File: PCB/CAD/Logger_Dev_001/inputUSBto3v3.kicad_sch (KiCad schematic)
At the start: 22 parts, among them J4 Connector, USB-TYPE-C-16P, U4 MCP2221AxSL, U6 XC6206P332MR

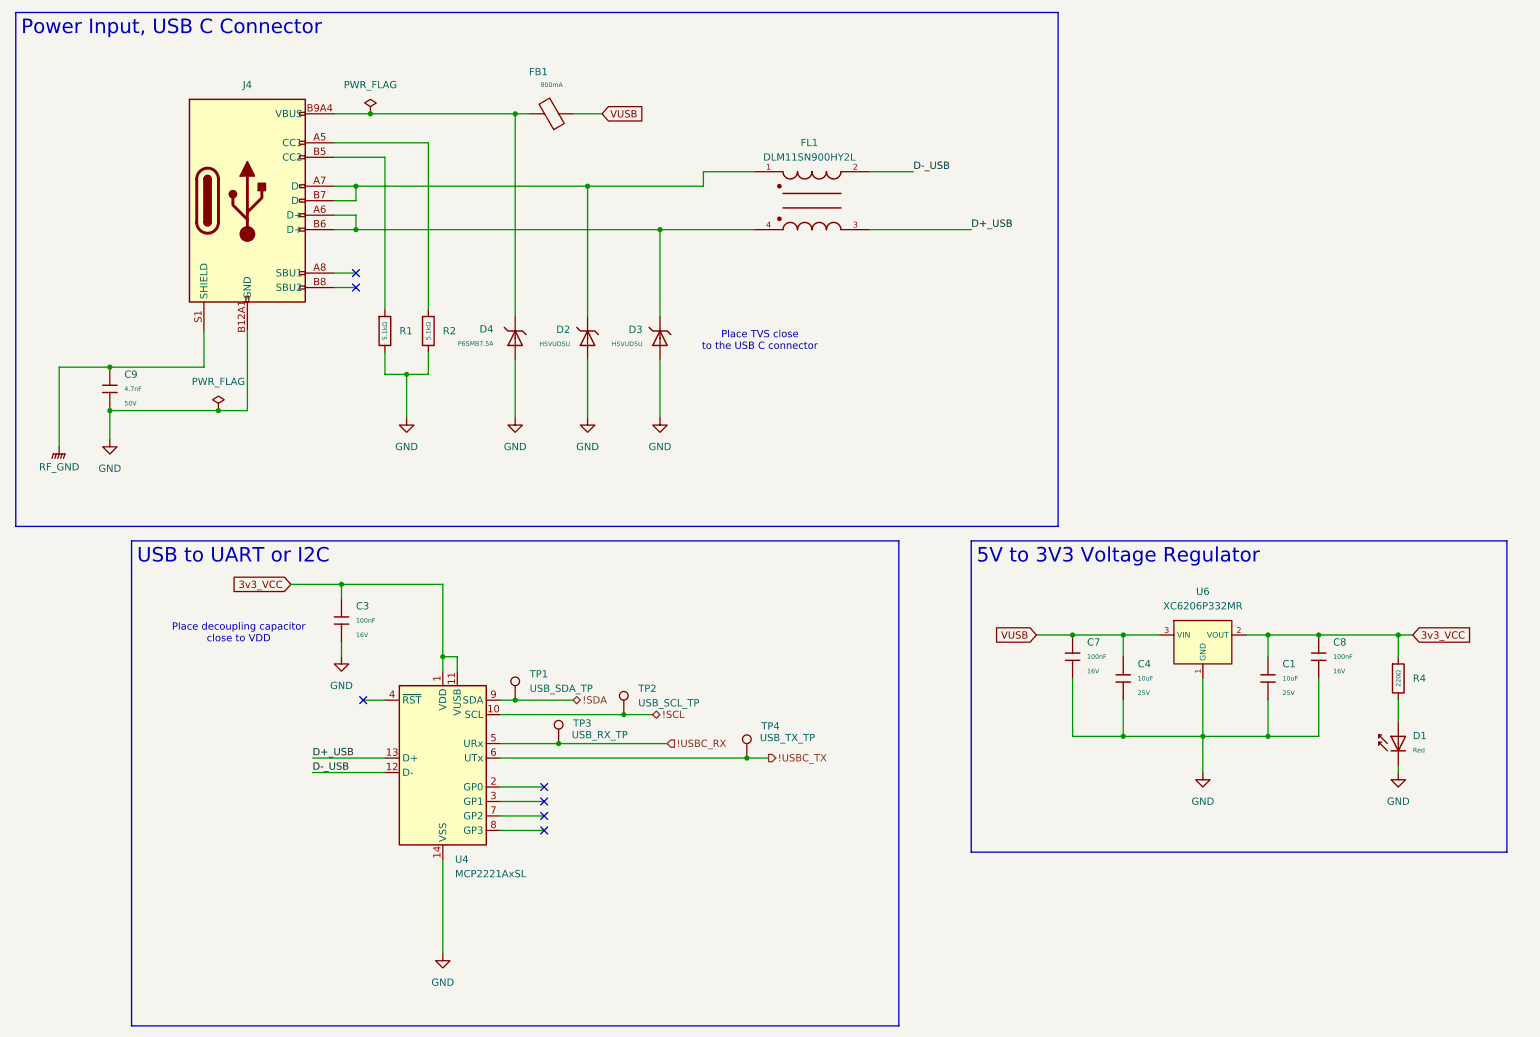
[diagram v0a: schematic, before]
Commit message: Updated Schematic
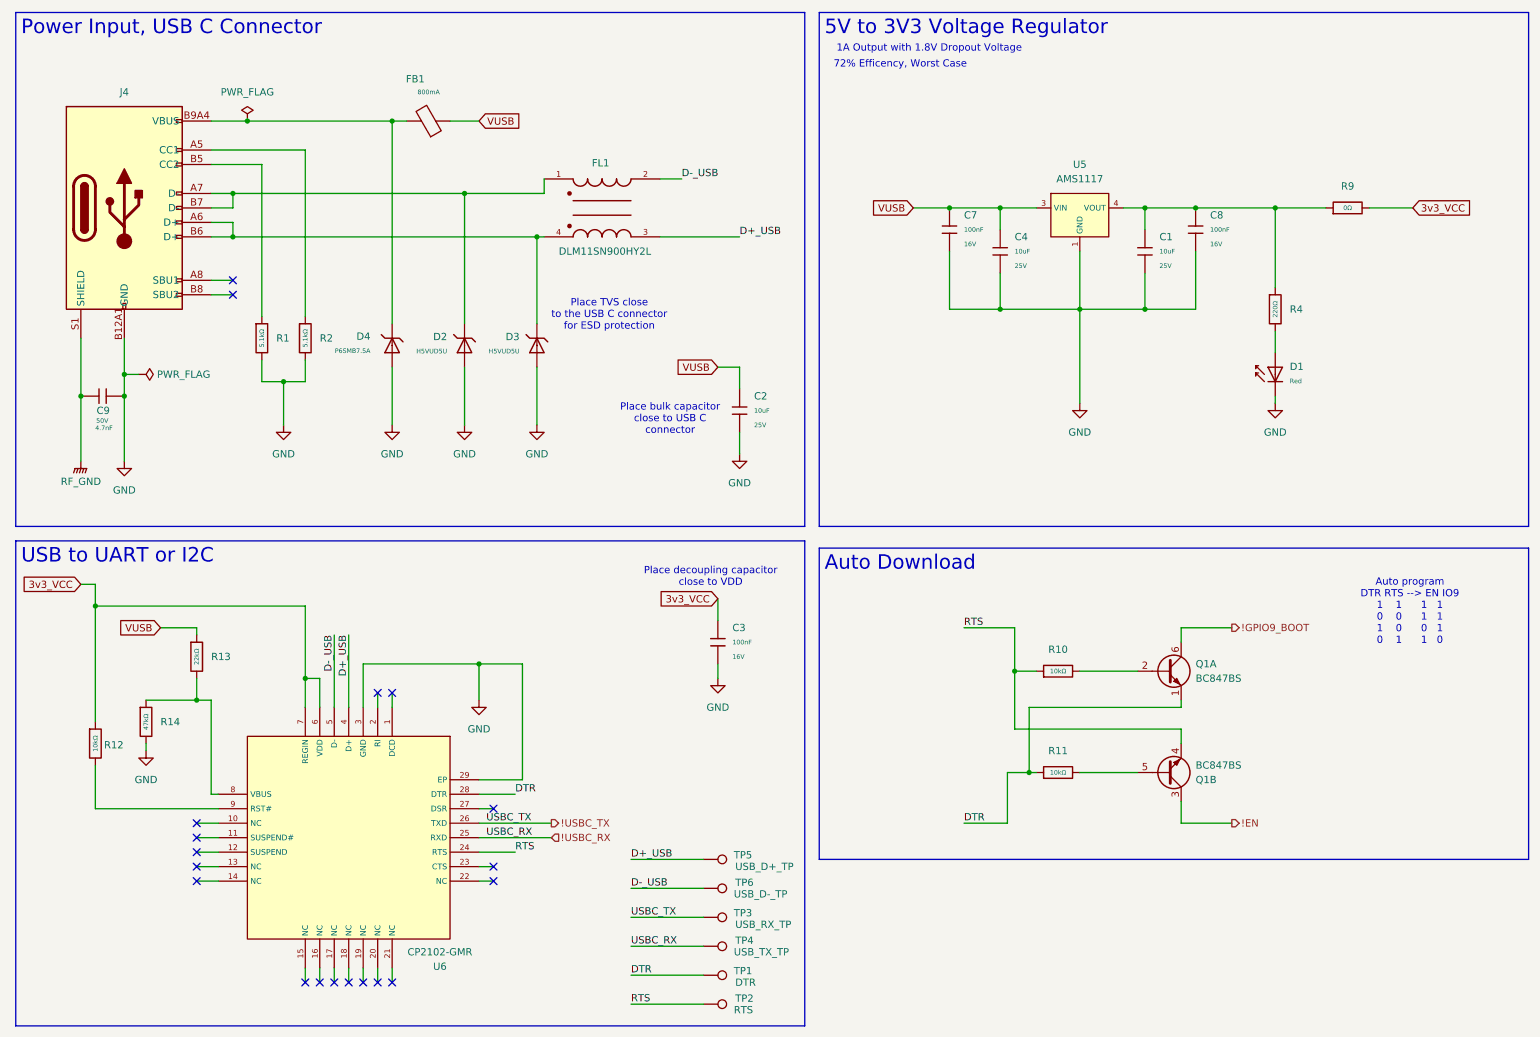
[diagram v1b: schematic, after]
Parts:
- removed U4: MCP2221AxSL, Package_SO:SOIC-14_3.9x8.7mm_P1.27mm, symbol Interface_USB:MCP2221AxSL
- removed U6: XC6206P332MR, PCM_JLCPCB:SOT-23-3_L2.9-W1.6-P1.90-LS2.8-BR, symbol PCM_JLCPCB-Power:LDO, 3.3V, 0.2A
- added C2: 10uF, PCM_JLCPCB:C_0603, symbol PCM_JLCPCB-Capacitors:0603,10uF,(2)
- added Q1: BC847BS, PCM_JLCPCB:SOT-363_SC-70-6, symbol PCM_JLCPCB-Transistor-Packages:NPN, 2 Channel, BC847BS
- added R10, R11, R12: 10kΩ, PCM_JLCPCB:R_0402, symbol PCM_JLCPCB-Resistors:0402,10kΩ
- added R13: 22kΩ, PCM_JLCPCB:R_0402, symbol PCM_JLCPCB-Resistors:0402,22kΩ
- added R14: 47kΩ, PCM_JLCPCB:R_0402, symbol PCM_JLCPCB-Resistors:0402,47kΩ
- added R9: 0Ω, PCM_JLCPCB:R_1206, symbol PCM_JLCPCB-Resistors:1206,0Ω
- added TP5: USB_D+_TP, symbol Connector:TestPoint
- added TP6: USB_D-_TP, symbol Connector:TestPoint
- added U5: AMS1117, PCM_JLCPCB:SOT-223-3_L6.5-W3.4-P2.30-LS7.0-BR, symbol PCM_JLCPCB-Power:LDO, 3.3V, 1A
- added U6: CP2102-GMR, PCM_JLCPCB:WQFN-28_L5.0-W5.0-P0.50-BL-EP3.2, symbol PCM_JLCPCB-Interface:Transceiver, USB
- TP1: value USB_SDA_TP -> DTR
- TP2: value USB_SCL_TP -> RTS
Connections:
- net !USBC_RX: now also TP4.1, U6.25 (RXD); no longer TP3.1
- net !USBC_TX: now also TP3.1, U6.26 (TXD); no longer TP4.1
- net 3v3_VCC: now also R12.1, R9.2, U6.6 (VDD), U6.7 (REGIN); no longer C1.1, C8.1, R4.1
- net D+_USB: now also TP5.1, U6.4 (D+)
- net D-_USB: now also TP6.1, U6.5 (D-)
- net GND: now also C2.2, R14.2, U5.1 (GND), U6.29 (EP), U6.3 (GND)
- net VUSB: now also C2.1, R13.1, U5.3 (VIN)
- net !SCL renamed RTS
- net RTS: now also Q1.4 (E2), R10.1, U6.24 (RTS)
- net !SDA renamed DTR
- net DTR: now also Q1.1 (E1), R11.1, U6.28 (DTR)
- new net: C1.1, C8.1, R4.1, R9.1, U5.2 (VOUT), U5.4 (VOUT)
- new net: Q1.2 (B1), R10.2
- new net: R12.2, U6.9 (RST#)
- new net: R13.2, R14.1, U6.8 (VBUS)
- new net: Q1.5 (B2), R11.2
- new net !EN: Q1.3 (C2)
- new net !GPIO9_BOOT: Q1.6 (C1)
- no-connect marks 7 -> 19
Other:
- note added: "1A Output with 1.8V Dropout Voltage"
- note added: "72% Efficency, Worst Case"
- note added: "Auto program DTR RTS --> EN IO9 1 1 1 1 0 0 1 1 1 0 0 1 0 1 1 0"
- note added: "Place TVS close to the USB C connector for ESD protection"
- note added: "Place bulk capacitor close to USB C connector"
- note removed: "Place TVS close to the USB C connector"
- company: (none) -> Jake Odgers
- title: (none) -> Mileage Logger
- moved on the sheet: C1, C3, C4, C7, C8, C9, D1, D2, D3, D4, FB1, FL1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
